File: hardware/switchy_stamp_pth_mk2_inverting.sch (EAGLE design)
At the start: 20 parts, among them IC1 MC34063

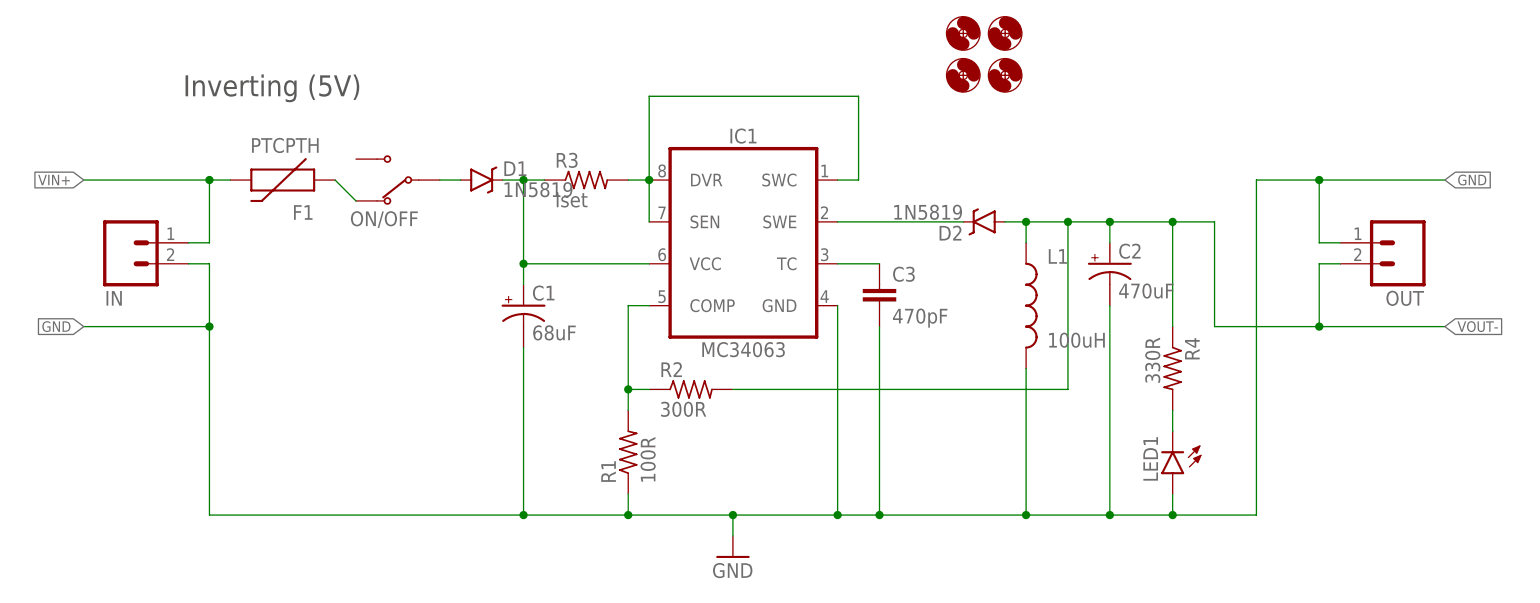
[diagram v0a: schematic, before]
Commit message: fixed a few mistakes, still rearranging
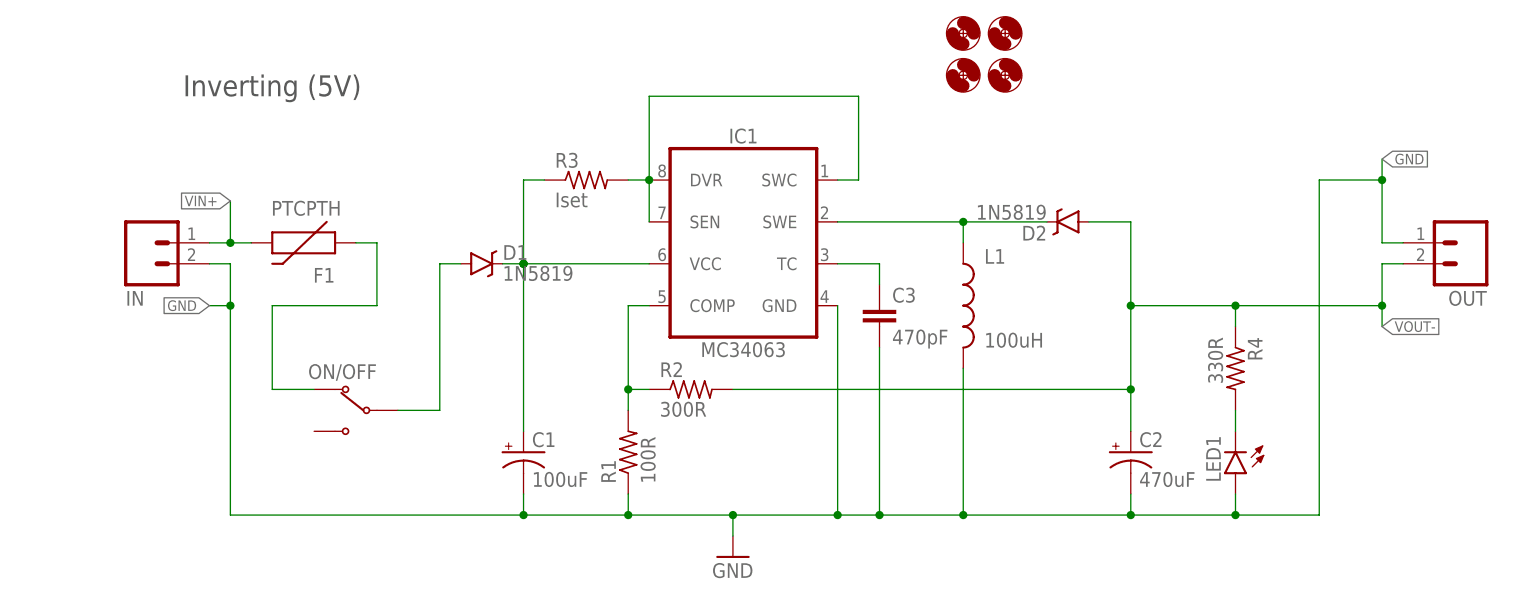
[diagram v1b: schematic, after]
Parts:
- C1: value 68uF -> 100uF
- H1, H2, H3, H4: value HOLE#4 -> HOLE#2; device A_butts:HOLE#4 -> A_butts:HOLE#2
- L1: device A_butts:INDUCTORRLB0912 -> A_butts:INDUCTORRADIAL-PTH-3-BY-6.7DIA
- ON/OFF: value SWITCH-SPDTPTH-RA-2.54MM -> SWITCH-SPDTPTH-VERT-2.54MM; device A_butts:SWITCH-SPDTPTH-RA-2.54MM -> A_butts:SWITCH-SPDTPTH-VERT-2.54MM
- R3: device A_butts:RESISTOR -> A_butts:RESISTORAXIAL-PTH-7.68MM
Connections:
- net N$6: now also L1.1
- net VOUT-: no longer L1.1
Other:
- moved on the sheet: C1, C2, C3, D1, D2, F1, IN, L1, LED1, ON/OFF, OUT, R4
